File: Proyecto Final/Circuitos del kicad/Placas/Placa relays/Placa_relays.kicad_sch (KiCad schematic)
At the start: 47 parts, among them J1 12v, J4 Conn_01x08, J5 Conn_01x08, J6 Conn_01x06, Q1 PN2222A, Q2 PN2222A, Q3 PN2222A, SW1 SW_Push, SW2 SW_Push, SW3 SW_Push, SW4 SW_Push, U1 LM7805, U2 ESP-12E, U3 ATmega328P-P, U4 LM1117-3.3, U5 BOB-12009, Y1 16MHz

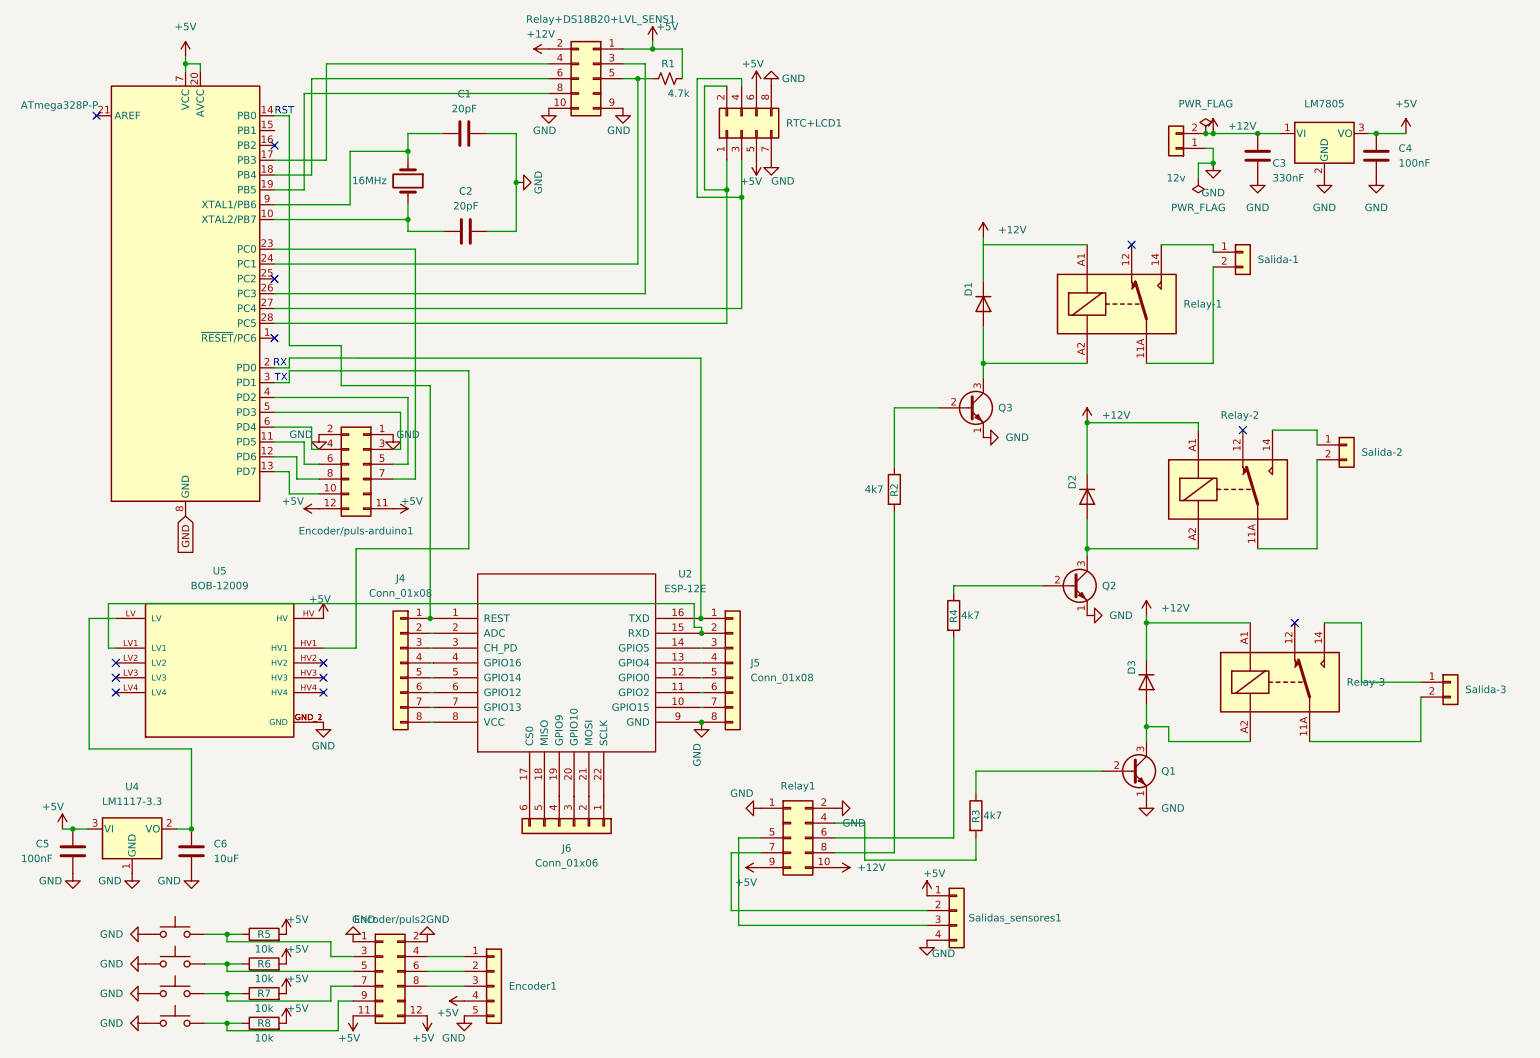
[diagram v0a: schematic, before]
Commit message: Cambios placa relays
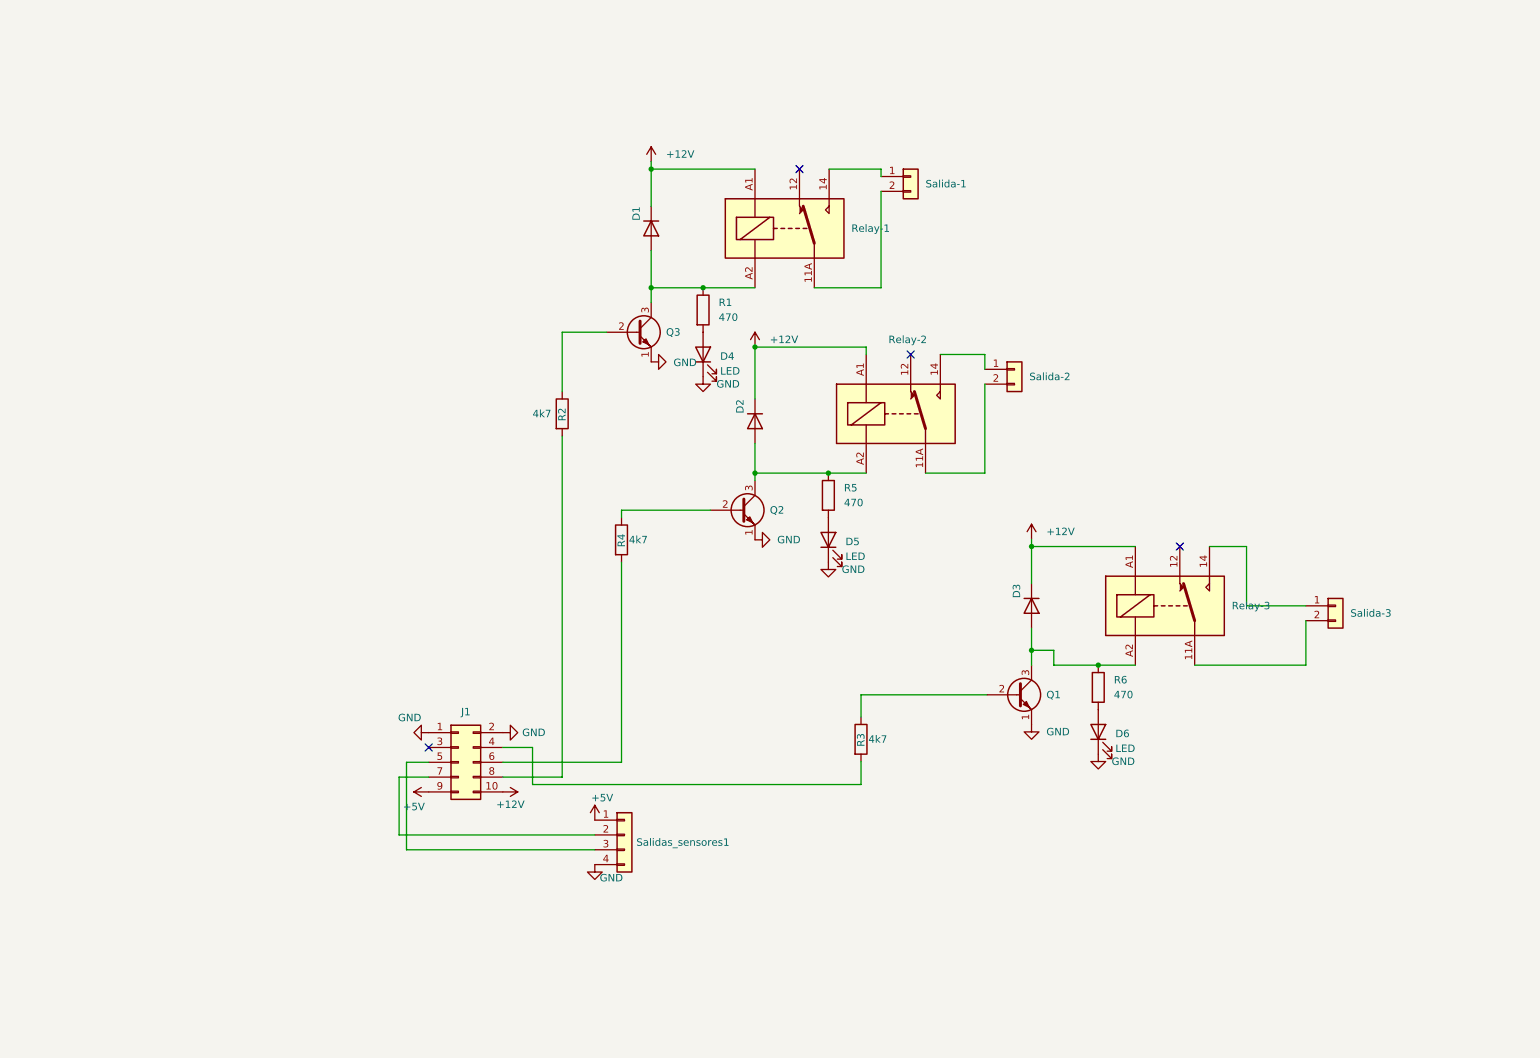
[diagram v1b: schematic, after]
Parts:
- removed C1, C2: 20pF, Capacitor_THT:C_Disc_D5.0mm_W2.5mm_P5.00mm, symbol Device:C
- removed C3: 330nF, Capacitor_THT:C_Disc_D5.0mm_W2.5mm_P5.00mm, symbol Device:C
- removed C4, C5: 100nF, Capacitor_THT:C_Disc_D5.0mm_W2.5mm_P5.00mm, symbol Device:C
- removed C6: 10uF, Capacitor_THT:C_Disc_D5.0mm_W2.5mm_P5.00mm, symbol Device:C
- removed Encoder/puls-arduino1: Conn_02x06_Odd_Even, ENCODER+PULS:ENCODER+PULS_arduino, symbol ENCODER+PULS_arduino:Conn_02x06_Odd_Even
- removed Encoder/puls2: Conn_02x06_Odd_Even, ENCODER+PULS:ENCODER+PULS, symbol ENCODER+PULS:Conn_02x06_Odd_Even
- removed Encoder1: Conn_01x05, Connector_PinHeader_2.54mm:PinHeader_1x05_P2.54mm_Vertical, symbol Connector_Generic:Conn_01x05
- removed J1: 12v, TerminalBlock:TerminalBlock_bornier-2_P5.08mm, symbol Connector_Generic:Conn_01x02
- removed J4, J5: Conn_01x08, Connector_PinHeader_2.54mm:PinHeader_1x08_P2.54mm_Vertical, symbol Connector_Generic:Conn_01x08
- removed J6: Conn_01x06, Connector_PinHeader_2.54mm:PinHeader_1x06_P2.54mm_Vertical, symbol Connector_Generic:Conn_01x06
- removed R1: 4.7k, Resistor_THT:R_Axial_DIN0204_L3.6mm_D1.6mm_P5.08mm_Horizontal, symbol Device:R_Small_US
- removed R7, R8: 10k, Resistor_THT:R_Axial_DIN0204_L3.6mm_D1.6mm_P5.08mm_Horizontal, symbol Device:R
- removed RTC+LCD1: Conn_02x04_Odd_Even, Connector_PinHeader_2.54mm:PinHeader_2x04_P2.54mm_Vertical, symbol Connector_Generic:Conn_02x04_Odd_Even
- removed Relay+DS18B20+LVL_SENS1: Conn_02x05_Odd_Even_1, RELAY+DS18B20+LVLSENS:RELAY+DS18B20+LVLSENS, symbol RELAY+DS18B20+LVLSENS:Conn_02x05_Odd_Even_1
- removed Relay1: Conn_02x05_Odd_Even, RELAY+DS18B20+LVLSENS:ENCODER+PULS_PLACA_SALIDAS, symbol RELAY+DS18B20+LVLSENS_PLACA_SALIDAS:Conn_02x05_Odd_Even
- removed SW1, SW2, SW3, SW4: SW_Push, Button_Switch_THT:SW_PUSH-12mm, symbol Switch:SW_Push
- removed U1: LM7805, Package_TO_SOT_THT:TO-220-3_Vertical, symbol Regulator_Linear:LM7805_TO220
- removed U2: ESP-12E, ESP8266-12E_ESP-12E:XCVR_ESP8266-12E_ESP-12E, symbol ESP8266:ESP-12E
- removed U3: ATmega328P-P, Package_DIP:DIP-28_W7.62mm, symbol MCU_Microchip_ATmega:ATmega328P-P
- removed U4: LM1117-3.3, Package_TO_SOT_SMD:SOT-223, symbol Regulator_Linear:LM1117-3.3
- removed U5: BOB-12009, CONV_BOB-12009, symbol BOB-12009:BOB-12009
- removed Y1: 16MHz, Crystal:Crystal_HC49-4H_Vertical, symbol Device:Crystal
- added D4, D5, D6: LED, LED_THT:LED_D5.0mm, symbol Device:LED
- added J1: Conn_02x05_Odd_Even, Connector_IDC:IDC-Header_2x05_P2.54mm_Vertical, symbol Connector_Generic:Conn_02x05_Odd_Even
- added R1: 470, Resistor_THT:R_Axial_DIN0204_L3.6mm_D1.6mm_P5.08mm_Horizontal, symbol Device:R
- R5, R6: value 10k -> 470
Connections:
- net +12V: now also J1.10 (Pin_10)
- net +5V: now also J1.9 (Pin_9); no longer R5.2, R6.2
- net GND: now also D4.1 (K), D5.1 (K), D6.1 (K), J1.1 (Pin_1), J1.2 (Pin_2)
- net at D1.2 (A), Q3.3 (C), Relay-1.A2: now also R1.1
- net at D3.2 (A), Q1.3 (C), Relay-3.A2: now also R6.1
- net at R3.2: now also J1.4 (Pin_4)
- net at D2.2 (A), Q2.3 (C), Relay-2.A2: now also R5.1
- net at R2.2: now also J1.8 (Pin_8)
- net at Salidas_sensores1.3 (Pin_3): now also J1.5 (Pin_5)
- net at R4.2: now also J1.6 (Pin_6)
- net at Salidas_sensores1.2 (Pin_2): now also J1.7 (Pin_7)
- new net: D5.2 (A), R5.2
- new net: D4.2 (A), R1.2
- new net: D6.2 (A), R6.2
- no-connect marks 13 -> 4
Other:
- note removed: "RST"
- note removed: "RX"
- note removed: "TX"
- moved on the sheet: D1, D2, D3, Q1, Q2, Q3, R2, R3, R4, Relay-1, Relay-2, Relay-3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
